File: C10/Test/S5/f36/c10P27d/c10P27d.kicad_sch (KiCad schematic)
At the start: 5 parts

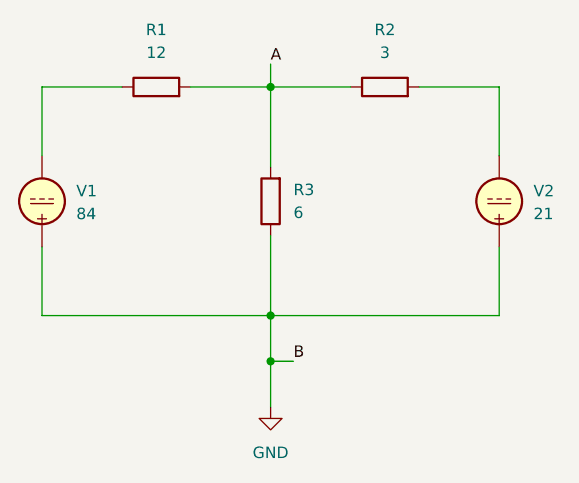
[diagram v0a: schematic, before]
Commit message: additiona upload Chapter 10
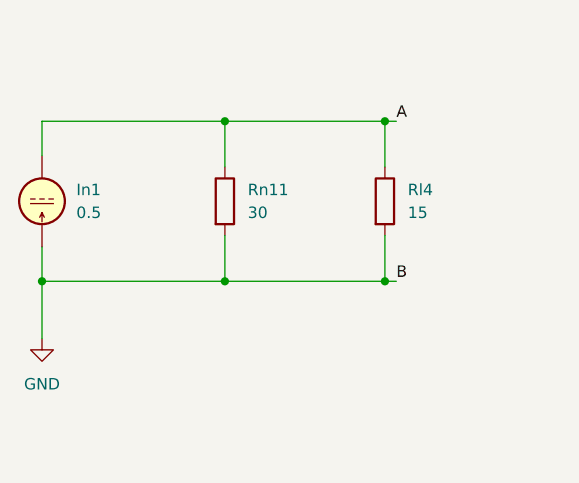
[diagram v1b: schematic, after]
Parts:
- removed R1: 12, symbol Device:R
- removed R2: 3, symbol Device:R
- removed R3: 6, symbol Device:R
- removed V1: 84, symbol Simulation_SPICE:VDC
- removed V2: 21, symbol Simulation_SPICE:VDC
- added In1: 0.5, symbol Simulation_SPICE:IDC
- added Rl4: 15, symbol Device:R
- added Rn11: 30, symbol Device:R
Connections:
- net A: now also In1.2, Rl4.1, Rn11.1
- net GND: now also In1.1, Rl4.2, Rn11.2
